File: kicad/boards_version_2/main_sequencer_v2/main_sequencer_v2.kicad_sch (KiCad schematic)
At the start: 24 parts

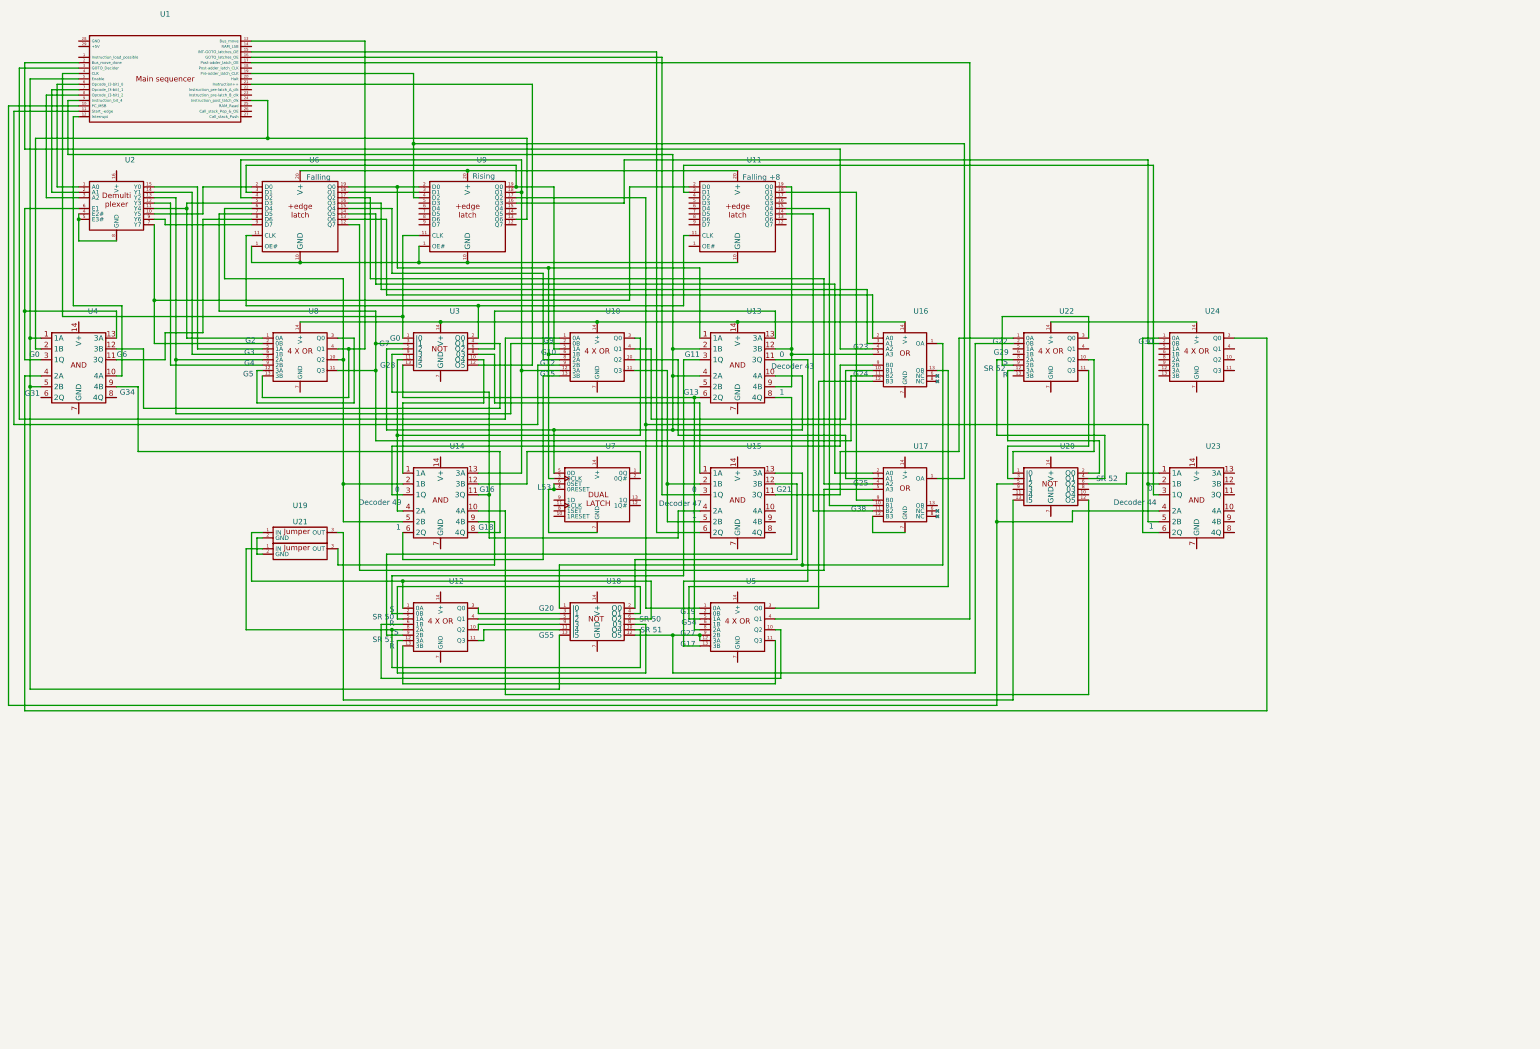
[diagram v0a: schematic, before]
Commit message: Sequencer almost checked
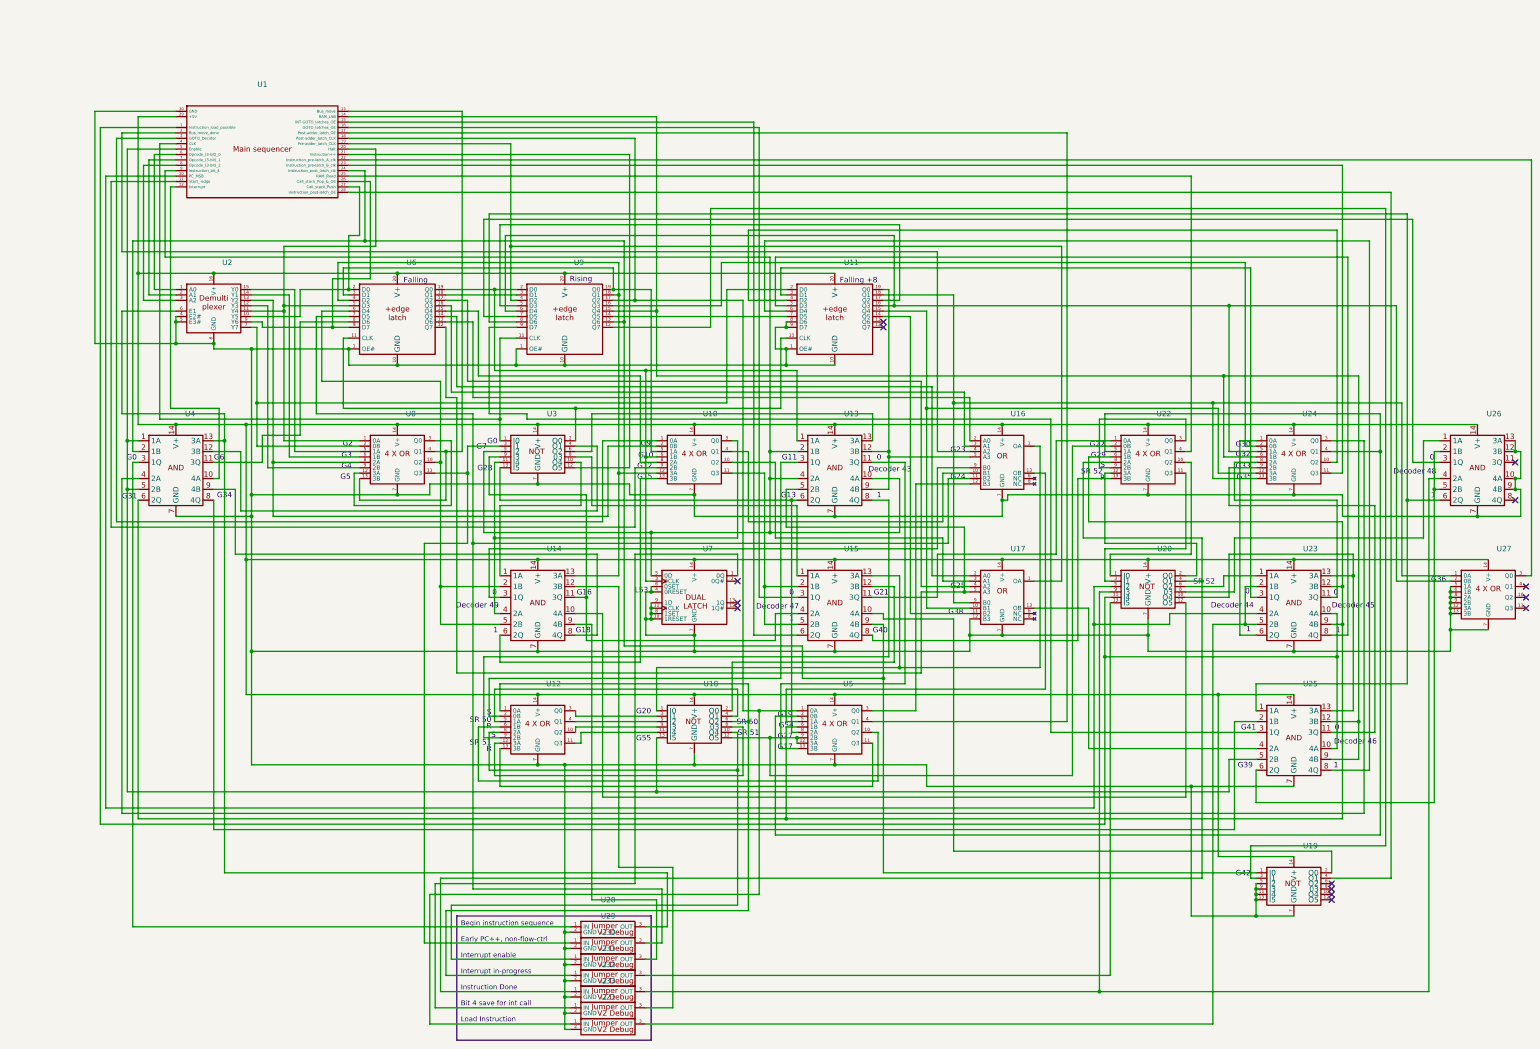
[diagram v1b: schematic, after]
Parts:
- removed U19, U21: ~, custom_footprint_library:jumper, symbol custom_symbol_lib:jumper
- added U19: ~, Package_DIP:DIP-14_W7.62mm, symbol custom_symbol_lib:6xNOT
- added U21, U28, U29, U30, U31, U32, U33: ~, custom_footprint_library:jumper_v2_gnd_debug_footprint, symbol custom_symbol_lib:jumper_v2_gnd_debug
- added U25, U26: ~, Package_DIP:DIP-14_W7.62mm, symbol custom_symbol_lib:quad_and
- added U27: ~, Package_DIP:DIP-14_W7.62mm, symbol custom_symbol_lib:quad_OR
- U1: footprint Connector_PinHeader_2.54mm:PinHeader_1x29_P2.54mm_Vertical -> Connector_PinHeader_2.54mm:PinHeader_1x30_P2.54mm_Vertical
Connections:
- net at U7.1 (0Q): now also U33.1 (IN); no longer U14.12 (3B)
- net at U7.10 (1RESET): now also U1.30 (GND), U10.7 (GND), U11.1 (OE#), U11.10 (GND), U11.8 (D6), U11.9 (D7), U12.7 (GND), U13.7 (GND), U14.7 (GND), U15.7 (GND), U16.7 (GND), U17.12 (B3), U17.7 (GND), U18.7 (GND), U2.4 (E2#), U2.5 (E3#), U2.8 (GND), U20.7 (GND), U22.7 (GND), U23.7 (GND), U24.7 (GND), U3.7 (GND), U4.7 (GND), U5.7 (GND), U6.1 (OE#), U6.10 (GND), U7.11 (1CLK), U7.4 (0RESET), U7.6 (0SET), U7.7 (GND), U7.8 (1SET), U7.9 (1D), U8.7 (GND), U9.1 (OE#), U9.10 (GND), U19.11 (I4), U19.13 (I5), U19.5 (I2), U19.7 (GND), U19.9 (I3), U21.2 (GND), U25.7 (GND), U26.10 (4A), U26.12 (3B), U26.13 (3A), U26.7 (GND), U26.9 (4B), U27.12 (3A), U27.13 (3B), U27.5 (1A), U27.6 (1B), U27.7 (GND), U27.8 (2A), U27.9 (2B), U28.2 (GND), U29.2 (GND), U30.2 (GND), U31.2 (GND), U32.2 (GND), U33.2 (GND)
- net at U7.14 (V+): now also U1.29 (+5V), U10.14 (V+), U11.20 (V+), U12.14 (V+), U13.14 (V+), U14.14 (V+), U15.14 (V+), U16.14 (V+), U17.14 (V+), U18.14 (V+), U2.16 (V+), U20.14 (V+), U22.14 (V+), U23.14 (V+), U24.14 (V+), U3.14 (V+), U4.14 (V+), U5.14 (V+), U6.20 (V+), U8.14 (V+), U9.20 (V+), U19.14 (V+), U25.14 (V+), U26.14 (V+), U27.14 (V+)
- net at U17.5 (A3), U6.12 (Q7): now also U13.5 (2B)
- net at U2.10 (Y5), U6.2 (D0): now also U1.27 (Call_stack_Push)
- net at U2.11 (Y4), U6.5 (D3), U8.1 (0A): now also U1.20 (Halt)
- net at U16.11 (B2), U6.7 (D5): now also U29.3 (OUT); no longer U3.3 (I1), U8.11 (Q3)
- net at U2.9 (Y6), U6.9 (D7): now also U1.26 (Call_stack_Pop_&_OE)
- net at U1.5 (Enable), U18.13 (I5), U4.1 (1A)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: now also U25.5 (2B)
- net at U2.6 (E1), U4.13 (3A): now also U28.3 (OUT); no longer U4.3 (1Q)
- net at U1.24 (Instruction_post_latch_clk), U4.2 (1B), U9.13 (Q6): now also U15.9 (4B), U19.1 (I0)
- net at U4.6 (2Q): now also U22.6 (1B), U23.12 (3B), U23.9 (4B), U5.6 (1B)
- net at U4.8 (4Q): now also U25.2 (1B)
- net at U12.8 (2A), U18.10 (O4): now also U30.1 (IN)
- net at U12.1 (0A), U18.6 (O2): now also U31.1 (IN)
- net at U15.10 (4A): now also U19.2 (O0)
- net at U15.8 (4Q): now also U22.13 (3B)
- net at U11.15 (Q4), U17.10 (B1): now also U24.12 (3A)
- net at U11.16 (Q3): now also U24.5 (1A), U9.6 (D4), U27.2 (0B)
- net at U11.17 (Q2): now also U9.5 (D3)
- net at U11.18 (Q1), U17.9 (B0): now also U24.13 (3B), U27.1 (0A)
- net at U11.4 (D2): now also U24.10 (Q2)
- net at U11.5 (D3): now also U23.8 (4Q)
- net at U11.6 (D4): now also U25.8 (4Q)
- net at U11.7 (D5): now also U9.14 (Q5)
- net at U23.10 (4A): now also U1.1 (Instruction_load_possible), U20.11 (I4), U25.10 (4A)
- net at U23.11 (3Q): now also U24.8 (2A)
- net at U23.13 (3A): now also U20.10 (O4), U25.13 (3A)
- net at U23.2 (1B), U23.5 (2B): now also U21.3 (OUT); no longer U5.1 (0A), U9.17 (Q2)
- net at U20.13 (I5): now also U31.3 (OUT)
- net at U1.14 (RAM_LSB): now also U24.6 (1B), U9.15 (Q4), U25.12 (3B), U25.9 (4B)
- net at U1.18 (Post-adder_latch_CLK): now also U5.1 (0A), U9.17 (Q2), U21.1 (IN)
- net at U1.22 (Instruction_pre-latch_A_clk): now also U27.3 (Q0)
- net at U1.23 (Instruction_pre-latch_B_clk): now also U24.11 (Q3)
- net at U1.25 (RAM_Read): now also U22.4 (Q1)
- net at U1.28 (Instruction_post-latch_OE): now also U19.4 (O1)
- net at U17.13 (OB): now also U25.4 (2A)
- net at U14.9 (4B): now also U30.3 (OUT)
- net at U24.4 (Q1): now also U22.5 (1A), U5.2 (0B)
- net at U24.9 (2B): now also U25.11 (3Q)
- net at U9.12 (Q7): now also U19.3 (I1)
- net at U9.7 (D5): now also U26.3 (1Q)
- net at U9.8 (D6): now also U25.1 (1A), U26.6 (2Q)
- net at U9.9 (D7): now also U25.3 (1Q)
- net at U20.4 (O1), U22.8 (2A): now also U32.1 (IN)
- net at U20.8 (03): now also U26.1 (1A)
- net at U20.9 (I3): now also U26.4 (2A), U32.3 (OUT)
- new net: U28.1 (IN), U4.3 (1Q)
- new net: U25.6 (2Q), U26.2 (1B), U26.5 (2B)
- new net: U29.1 (IN), U3.3 (I1), U8.11 (Q3)
- new net: U14.12 (3B), U33.3 (OUT)
- no-connect marks 0 -> 14
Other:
- note added: "Decoder 45"
- note added: "Decoder 46"
- note added: "Decoder 48"
- note added: "G32"
- note added: "G33"
- note added: "G35"
- note added: "G36"
- note added: "G39"
- note added: "G40"
- note added: "G41"
- note added: "G42"
- moved on the sheet: U10, U11, U12, U13, U14, U15, U16, U17, U18, U2, U20, U22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
